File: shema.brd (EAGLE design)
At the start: 53.6 x 25 mm, 20 parts

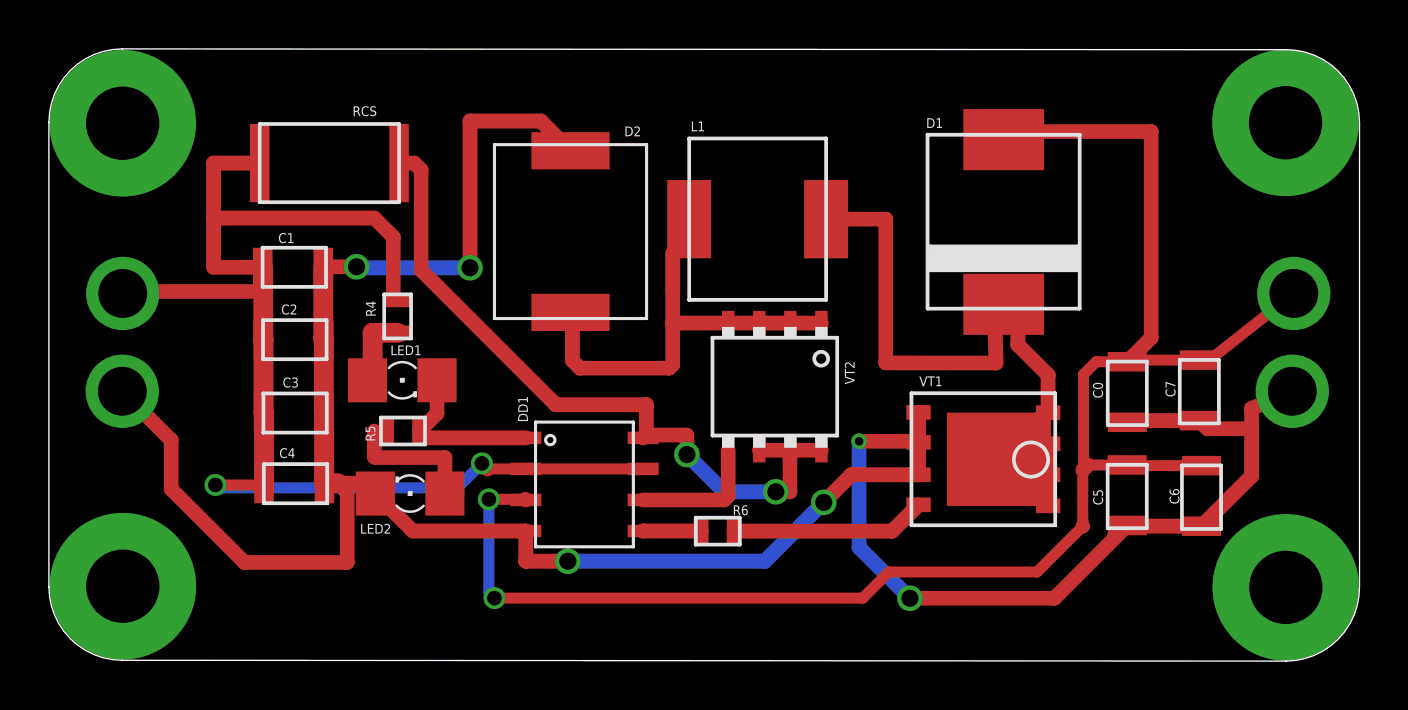
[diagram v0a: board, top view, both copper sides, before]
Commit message: изменения файлов
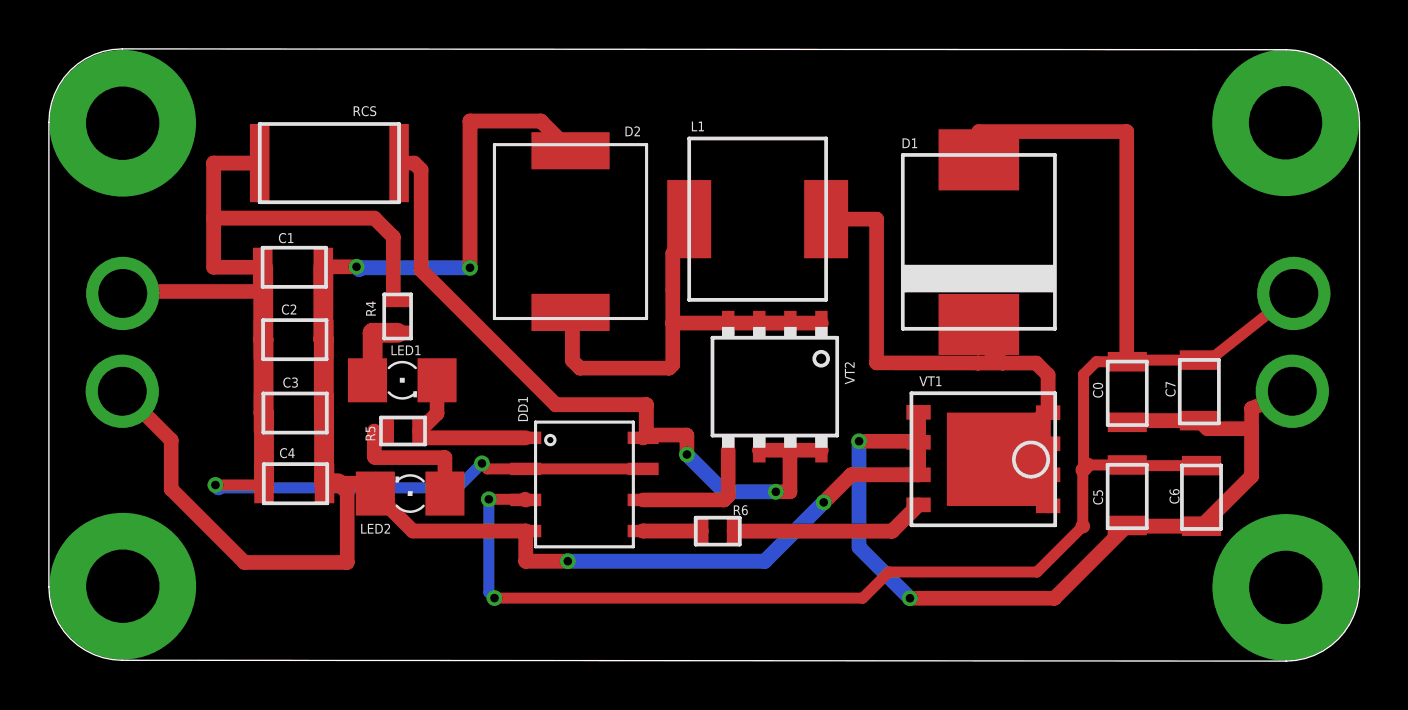
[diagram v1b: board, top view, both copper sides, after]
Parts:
- moved D1 1.31 mm to (38.0, 17.1)
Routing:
- net N$6: track 29.5 -> 27.2 mm
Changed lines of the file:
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@@
 <attribute name="VALUE" x="45.72" y="12.56" size="0.4064" layer="27" rot="R270"/>
 </element>
-<element name="D1" library="1_DIOD" package="CB417-15" value="B560C-13-F" x="39.041" y="17.935" smashed="yes" rot="R90">
-<attribute name="NAME" x="35.87" y="21.767" size="0.4" layer="25"/>
-<attribute name="VALUE" x="43.613" y="14.506" size="1.27" layer="27" rot="R90"/>
+<element name="D1" library="1_DIOD" package="CB417-15" value="B560C-13-F" x="38.029" y="17.109" smashed="yes" rot="R90">
+<attribute name="NAME" x="34.858" y="20.941" size="0.4" layer="25"/>
+<attribute name="VALUE" x="42.601" y="13.68" size="1.27" layer="27" rot="R90"/>
 </element>
 <element name="D2" library="1_DIOD" package="DIOD" value="SS36C" x="21.33" y="17.53" smashed="yes" rot="R270">
@@
 <wire x1="24.3" y1="7.825" x2="19.5" y2="7.825" width="0.45" layer="1"/>
 <wire x1="19.5" y1="7.825" x2="17.9326" y2="7.825" width="0.45" layer="1"/>
-<wire x1="17.7076" y1="8.05" x2="17.9326" y2="7.825" width="0.6096" layer="1"/>
-<via x="17.7076" y="8.05" extent="1-16" drill="0.6" diameter="0.44"/>
+<wire x1="17.7076" y1="8.05" x2="17.9326" y2="7.825" width="0.45" layer="1"/>
+<via x="17.7076" y="8.05" extent="1-16" drill="0.35"/>
 <wire x1="17.7076" y1="8.05" x2="16.7076" y2="7.05" width="0.45" layer="16"/>
-<via x="6.81" y="7.168" extent="1-16" drill="0.6" diameter="0.55"/>
+<via x="6.81" y="7.168" extent="1-16" drill="0.35"/>
 <wire x1="13.3112625" y1="18.08" x2="6.736" y2="18.08" width="0.6096" layer="1"/>
 <wire x1="8.746" y1="16.07" x2="6.736" y2="16.07" width="0.6" layer="1"/>
@@
 <contactref element="VT1" pad="P$4"/>
 <contactref element="VT1" pad="P$9"/>
-<wire x1="39.6235" y1="14.05" x2="38.6755625" y2="14.05" width="0.6096" layer="1"/>
-<wire x1="38.6755625" y1="14.05" x2="38.535" y2="14.05" width="0.6096" layer="1"/>
-<wire x1="38.7305125" y1="12.1538125" x2="34.22" y2="12.160478125" width="0.6" layer="1"/>
-<wire x1="34.22" y1="12.160478125" x2="34.22" y2="18.038" width="0.6" layer="1"/>
+<wire x1="33.845" y1="12.16103125" x2="38.000228125" y2="12.154890625" width="0.6" layer="1"/>
+<wire x1="33.845" y1="12.16103125" x2="33.845" y2="18.038" width="0.6" layer="1"/>
 <wire x1="40.86" y1="6.315" x2="40.86" y2="7.585" width="0.6096" layer="1"/>
 <wire x1="40.86" y1="7.585" x2="40.86" y2="8.855" width="0.6096" layer="1"/>
 <wire x1="38.845" y1="8.22" x2="40.75" y2="10.125" width="0.6096" layer="1"/>
 <wire x1="40.75" y1="10.125" x2="40.86" y2="10.125" width="0.6096" layer="1"/>
-<wire x1="39.6235" y1="14.05" x2="39.6235" y2="12.9015" width="0.6096" layer="1"/>
 <wire x1="40.86" y1="10.125" x2="40.86" y2="11.665" width="0.6096" layer="1"/>
-<wire x1="40.86" y1="11.665" x2="39.6235" y2="12.9015" width="0.6096" layer="1"/>
-<wire x1="34.22" y1="18.038" x2="31.782" y2="18.038" width="0.6" layer="1"/>
-<wire x1="38.6755625" y1="14.05" x2="38.7305125" y2="12.1538125" width="0.6096" layer="1"/>
-<wire x1="39.041" y1="14.556" x2="38.535" y2="14.05" width="0.6096" layer="1"/>
+<wire x1="33.845" y1="18.038" x2="31.782" y2="18.038" width="0.6" layer="1"/>
 <wire x1="40.225" y1="8.22" x2="40.86" y2="8.855" width="0.6" layer="1"/>
 <wire x1="38.845" y1="8.22" x2="40.225" y2="8.22" width="0.6" layer="1"/>
 <wire x1="40.225" y1="8.22" x2="40.86" y2="7.585" width="0.6" layer="1"/>
+<wire x1="40.86" y1="11.665" x2="40.3711875" y2="12.1538125" width="0.6" layer="1"/>
+<wire x1="40.3711875" y1="12.1538125" x2="39" y2="12.1538125" width="0.6" layer="1"/>
+<wire x1="39" y1="12.1538125" x2="38.029" y2="13.1248125" width="0.6" layer="1"/>
+<wire x1="38.029" y1="13.1248125" x2="38.029" y2="13.73" width="0.6" layer="1"/>
+<wire x1="38.000228125" y1="12.154890625" x2="38.00130625" y2="12.1538125" width="0.6" layer="1"/>
+<wire x1="38.00130625" y1="12.1538125" x2="39" y2="12.1538125" width="0.6" layer="1"/>
 </signal>
 <signal name="GND">
@@
 <wire x1="11.82" y1="7.24" x2="11.251" y2="7.24" width="0.8128" layer="1"/>
 <wire x1="19.5" y1="5.285" x2="14.882" y2="5.285" width="0.6096" layer="1"/>
-<via x="31.685" y="6.4564" extent="1-16" drill="0.7" diameter="0.55"/>
+<via x="31.685" y="6.4564" extent="1-16" drill="0.35"/>
 <wire x1="31.685" y1="6.4564" x2="29.2786" y2="4.05" width="0.6096" layer="16"/>
 <wire x1="29.2786" y1="4.05" x2="21.22" y2="4.05" width="0.6096" layer="16"/>
-<via x="21.22" y="4.05" extent="1-16" drill="0.7" diameter="0.55"/>
+<via x="21.22" y="4.05" extent="1-16" drill="0.35"/>
 <wire x1="21.22" y1="4.05" x2="19.5" y2="4.05" width="0.6096" layer="1"/>
 <wire x1="19.5" y1="4.05" x2="19.5" y2="5.285" width="0.6096" layer="1"/>
@@
 <wire x1="44.095" y1="5.511" x2="41.119" y2="2.535" width="0.6" layer="1"/>
 <wire x1="41.119" y1="2.535" x2="35.21" y2="2.535" width="0.6" layer="1"/>
-<via x="35.21" y="2.535" extent="1-16" drill="0.7" diameter="0.55"/>
+<via x="35.21" y="2.535" extent="1-16" drill="0.35"/>
 <wire x1="33.13" y1="4.615" x2="33.13" y2="8.955" width="0.6" layer="16"/>
 <wire x1="35.21" y1="2.535" x2="33.13" y2="4.615" width="0.6096" layer="16"/>
@@
 <wire x1="13.35" y1="6.817" x2="12.927" y2="7.24" width="0.6096" layer="1"/>
 <wire x1="12.927" y1="7.24" x2="11.82" y2="7.24" width="0.6" layer="1"/>
-<via x="17.22" y="16.05" extent="1-16" drill="0.7" diameter="0.55"/>
+<via x="17.22" y="16.05" extent="1-16" drill="0.35"/>
 <wire x1="17.22" y1="16.05" x2="12.75" y2="16.05" width="0.6096" layer="16"/>
 <wire x1="12.75" y1="16.05" x2="12.685" y2="15.985" width="0.6096" layer="16"/>
 <wire x1="12.685" y1="15.985" x2="12.58" y2="16.09" width="0.6096" layer="16"/>
-<via x="12.58" y="16.09" extent="1-16" drill="0.7" diameter="0.55"/>
+<via x="12.58" y="16.09" extent="1-16" drill="0.35"/>
 <wire x1="11.221" y1="16.07" x2="11.241" y2="16.09" width="0.6096" layer="1"/>
 <wire x1="12.58" y1="16.09" x2="11.241" y2="16.09" width="0.6" layer="1"/>
@@
 <wire x1="47.043" y1="12.274" x2="44.165" y2="12.274" width="0.45" layer="1"/>
 <wire x1="44.165" y1="12.274" x2="44.097" y2="12.206" width="0.6096" layer="1"/>
-<wire x1="45.075" y1="13.184" x2="45.075" y2="21.62" width="0.6" layer="1"/>
-<wire x1="44.097" y1="12.206" x2="45.075" y2="13.184" width="0.6" layer="1"/>
-<wire x1="39.041" y1="21.62" x2="39.041" y2="21.29" width="0.6096" layer="1"/>
+<wire x1="44.075" y1="21.62" x2="44.075" y2="12.228" width="0.6" layer="1"/>
+<wire x1="44.097" y1="12.206" x2="44.075" y2="12.228" width="0.6" layer="1"/>
+<wire x1="38.029" y1="21.62" x2="38.029" y2="20.464" width="0.6096" layer="1"/>
 <wire x1="47.133" y1="7.958" x2="44.123" y2="7.958" width="0.45" layer="1"/>
 <wire x1="44.095" y1="7.986" x2="44.123" y2="7.958" width="0.45" layer="1"/>
@@
 <wire x1="19.5" y1="6.555" x2="19.472925" y2="6.582075" width="0.6096" layer="1"/>
 <wire x1="19.472925" y1="6.582075" x2="17.9906" y2="6.582075" width="0.45" layer="1"/>
-<via x="17.9906" y="6.582075" extent="1-16" drill="0.6" diameter="0.55"/>
+<via x="17.9906" y="6.582075" extent="1-16" drill="0.35"/>
 <wire x1="17.9906" y1="6.582075" x2="17.9906" y2="2.7716" width="0.45" layer="16"/>
 <wire x1="18.001" y1="2.7612" x2="18.22" y2="2.5422" width="0.45" layer="16"/>
-<via x="18.22" y="2.5422" extent="1-16" drill="0.6" diameter="0.55"/>
+<via x="18.22" y="2.5422" extent="1-16" drill="0.35"/>
 <wire x1="18.22" y1="2.5422" x2="33.283275" y2="2.5422" width="0.45" layer="1"/>
 <wire x1="33.283275" y1="2.5422" x2="34.350475" y2="3.6094" width="0.45" layer="1"/>
@@
 <wire x1="42.2782" y1="5.47961875" x2="40.40798125" y2="3.6094" width="0.45" layer="1"/>
 <wire x1="17.9906" y1="2.7716" x2="18.001" y2="2.7612" width="0.1524" layer="16"/>
-<wire x1="45.075" y1="21.62" x2="39.041" y2="21.62" width="0.6" layer="1"/>
+<wire x1="44.075" y1="21.62" x2="38.029" y2="21.62" width="0.6" layer="1"/>
 <wire x1="42.309" y1="11.689" x2="42.309" y2="7.808" width="0.45" layer="1"/>
 <wire x1="42.277" y1="7.776" x2="42.277" y2="5.48081875" width="0.45" layer="1"/>
@@
 <wire x1="31.589" y1="8.589" x2="30.319" y2="8.589" width="0.6" layer="1"/>
 <wire x1="30.319" y1="8.589" x2="30.304" y2="8.589" width="0.6" layer="1"/>
-<via x="29.727" y="6.889" extent="1-16" drill="0.7" diameter="0.55"/>
+<via x="29.727" y="6.889" extent="1-16" drill="0.35"/>
 <wire x1="30.304" y1="8.589" x2="29.049" y2="8.589" width="0.6" layer="1"/>
 <wire x1="29.727" y1="6.889" x2="27.613" y2="6.889" width="0.6" layer="16"/>
 <wire x1="27.613" y1="6.889" x2="26.09" y2="8.412" width="0.6" layer="16"/>
-<via x="26.09" y="8.412" extent="1-16" drill="0.7" diameter="0.55"/>
+<via x="26.09" y="8.412" extent="1-16" drill="0.35"/>
 <wire x1="26.09" y1="8.412" x2="26.09" y2="9.191" width="0.6" layer="1"/>
 <wire x1="26.09" y1="9.191" x2="26.071" y2="9.21" width="0.6" layer="1"/>
